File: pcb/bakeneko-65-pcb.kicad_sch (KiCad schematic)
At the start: 19 parts, among them J1 JST SH 4-pin, J2 AVR-ISP-6, SW1 Reset, U1 SRV05-4, U2 ATmega32U4-AU, U3 ATmega32U4-MU, Y1 16MHz

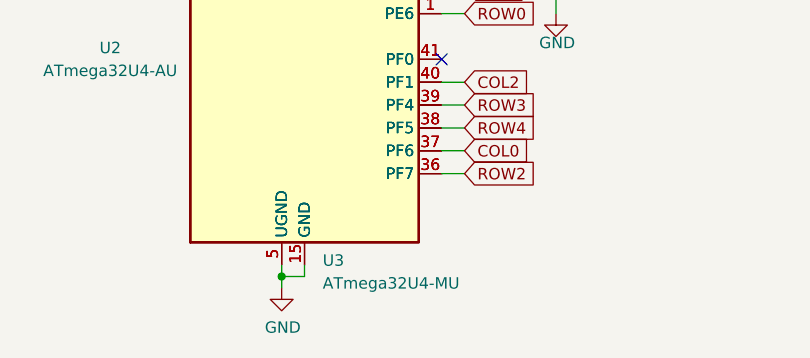
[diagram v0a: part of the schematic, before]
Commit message: Revert "Small updates - USB routing"
This reverts commit 01b81f097f4a432426e23b6d52fb9b838f85ddba.
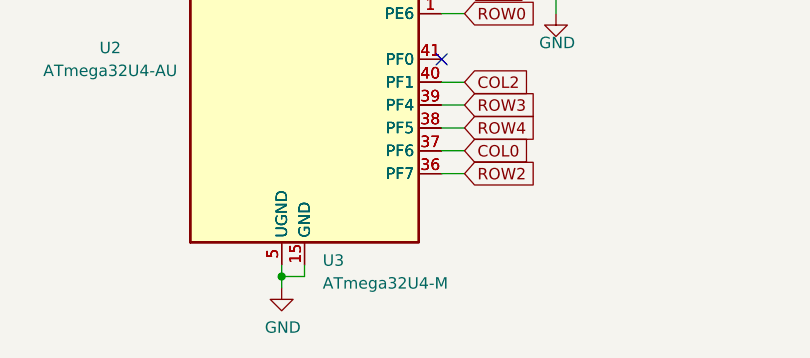
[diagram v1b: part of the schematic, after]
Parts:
- U3: value ATmega32U4-MU -> ATmega32U4-M; LCSC C112161 -> (none)
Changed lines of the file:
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@@
       (effects (font (size 1.27 1.27)) (justify left))
     )
-    (property "Value" "ATmega32U4-MU" (id 1) (at 60.4394 176.0173 0)
+    (property "Value" "ATmega32U4-M" (id 1) (at 60.4394 176.0173 0)
       (effects (font (size 1.27 1.27)) (justify left))
     )
@@
     )
     (property "Datasheet" "http://ww1.microchip.com/downloads/en/DeviceDoc/Atmel-7766-8-bit-AVR-ATmega16U4-32U4_Datasheet.pdf" (id 3) (at 58.42 128.27 0)
-      (effects (font (size 1.27 1.27)) hide)
-    )
-    (property "LCSC" "C112161" (id 4) (at 58.42 128.27 0)
       (effects (font (size 1.27 1.27)) hide)
     )
@@
     )
     (path "/d293ffd0-0d39-4336-b48b-d86bab8e7171"
-      (reference "U3") (unit 1) (value "ATmega32U4-MU") (footprint "Package_DFN_QFN:QFN-44-1EP_7x7mm_P0.5mm_EP5.2x5.2mm")
+      (reference "U3") (unit 1) (value "ATmega32U4-M") (footprint "Package_DFN_QFN:QFN-44-1EP_7x7mm_P0.5mm_EP5.2x5.2mm")
     )
     (path "/00000000-0000-0000-0000-00005f293f4e"

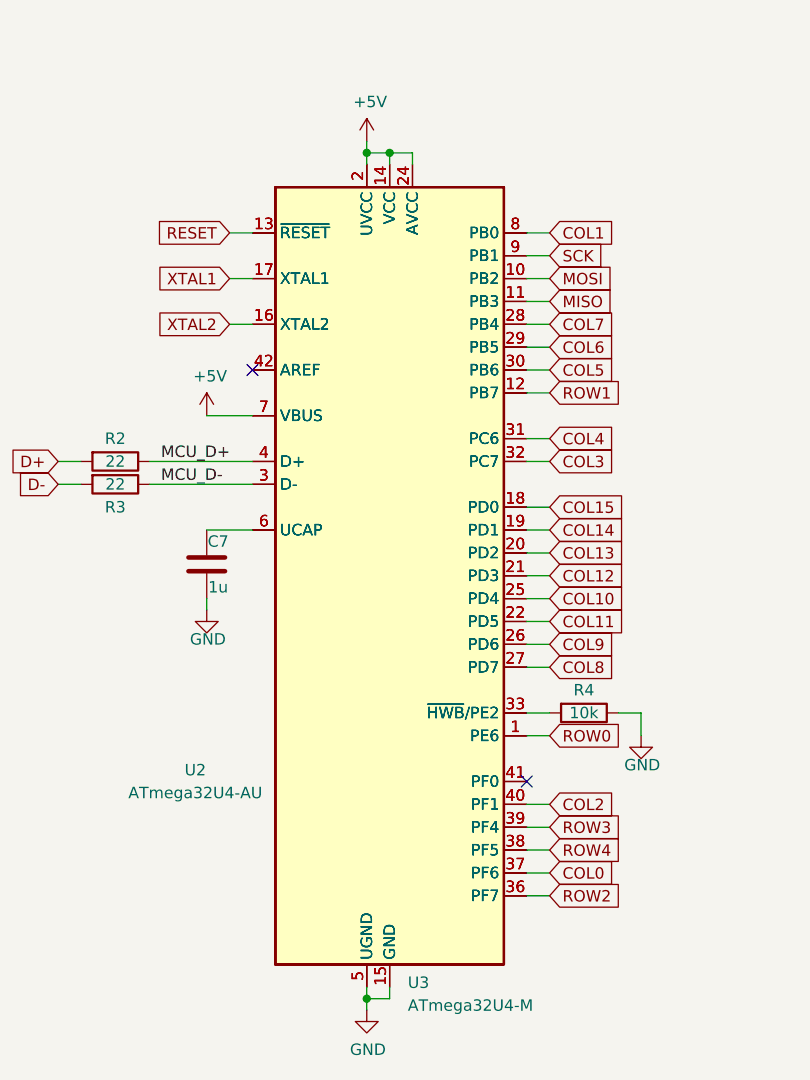
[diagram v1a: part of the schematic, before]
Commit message: Revert "Dual MCU footprint update"
This reverts commit d3ec1e4d8a5bc08a1e6c0b7459cdd594f23042e6.
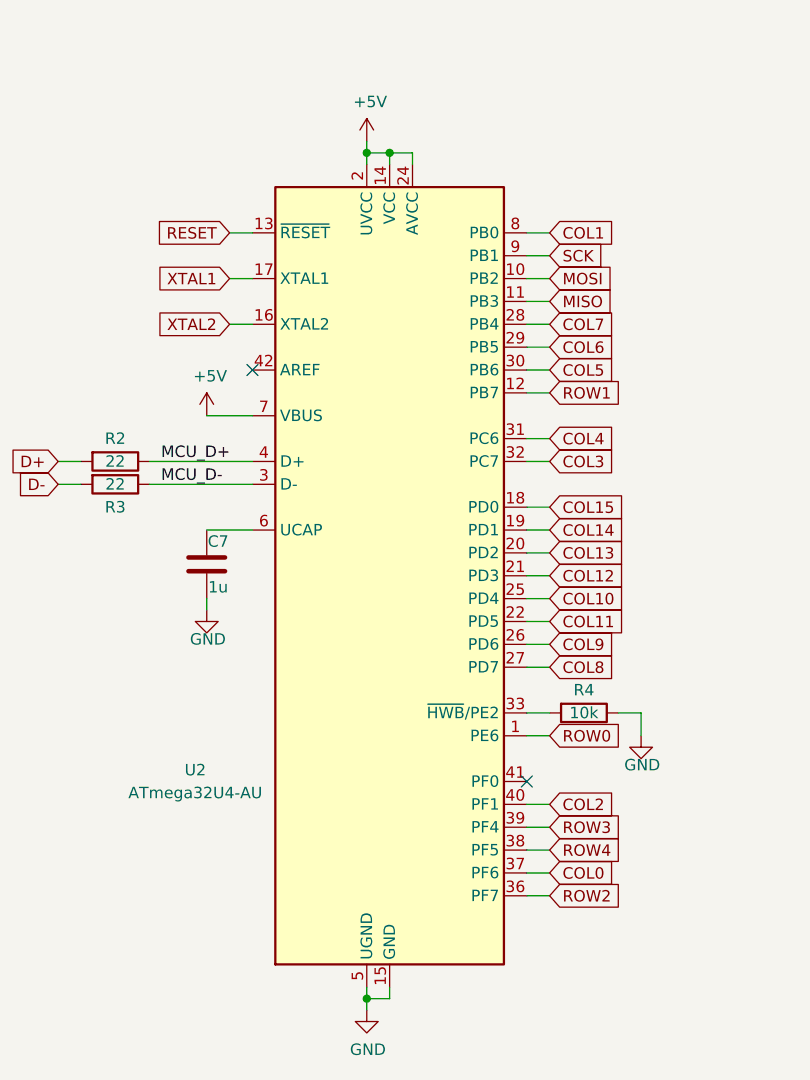
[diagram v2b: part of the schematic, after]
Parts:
- removed U3: ATmega32U4-M, Package_DFN_QFN:QFN-44-1EP_7x7mm_P0.5mm_EP5.2x5.2mm, symbol MCU_Microchip_ATmega:ATmega32U4-M
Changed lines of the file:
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@@
     (pin "1")
-  )
-  (symbol (lib_id "MCU_Microchip_ATmega:ATmega32U4-M") (at 58.42 128.27 0) (unit 1)
-    (in_bom yes) (on_board yes) (fields_autoplaced)
-    (property "Reference" "U3" (id 0) (at 60.4394 173.4804 0)
-      (effects (font (size 1.27 1.27)) (justify left))
-    )
-    (property "Value" "ATmega32U4-M" (id 1) (at 60.4394 176.0173 0)
-      (effects (font (size 1.27 1.27)) (justify left))
-    )
-    (property "Footprint" "Package_DFN_QFN:QFN-44-1EP_7x7mm_P0.5mm_EP5.2x5.2mm" (id 2) (at 58.42 128.27 0)
-      (effects (font (size 1.27 1.27) italic) hide)
-    )
-    (property "Datasheet" "http://ww1.microchip.com/downloads/en/DeviceDoc/Atmel-7766-8-bit-AVR-ATmega16U4-32U4_Datasheet.pdf" (id 3) (at 58.42 128.27 0)
-      (effects (font (size 1.27 1.27)) hide)
-    )
-    (pin "1")
-    (pin "10")
-    (pin "11")
-    (pin "12")
-    (pin "13")
-    (pin "14")
-    (pin "15")
-    (pin "16")
-    (pin "17")
-    (pin "18")
-    (pin "19")
-    (pin "2")
-    (pin "20")
-    (pin "21")
-    (pin "22")
-    (pin "23")
-    (pin "24")
-    (pin "25")
-    (pin "26")
-    (pin "27")
-    (pin "28")
-    (pin "29")
-    (pin "3")
-    (pin "30")
-    (pin "31")
-    (pin "32")
-    (pin "33")
-    (pin "34")
-    (pin "35")
-    (pin "36")
-    (pin "37")
-    (pin "38")
-    (pin "39")
-    (pin "4")
-    (pin "40")
-    (pin "41")
-    (pin "42")
-    (pin "43")
-    (pin "44")
-    (pin "45")
-    (pin "5")
-    (pin "6")
-    (pin "7")
-    (pin "8")
-    (pin "9")
   )
   (sheet (at 185.42 87.63) (size 45.72 53.34) (fields_autoplaced)
@@
       (reference "U2") (unit 1) (value "ATmega32U4-AU") (footprint "Package_QFP:TQFP-44_10x10mm_P0.8mm")
     )
-    (path "/d293ffd0-0d39-4336-b48b-d86bab8e7171"
-      (reference "U3") (unit 1) (value "ATmega32U4-M") (footprint "Package_DFN_QFN:QFN-44-1EP_7x7mm_P0.5mm_EP5.2x5.2mm")
-    )
     (path "/00000000-0000-0000-0000-00005f293f4e"
